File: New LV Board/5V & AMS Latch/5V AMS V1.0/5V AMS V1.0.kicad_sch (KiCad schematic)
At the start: 17 parts, among them J2 B12B-PH-K-S, J4 691137710002, K1 AHES4291, SW1 Test Reset AMS, U1 LT1117-5.0

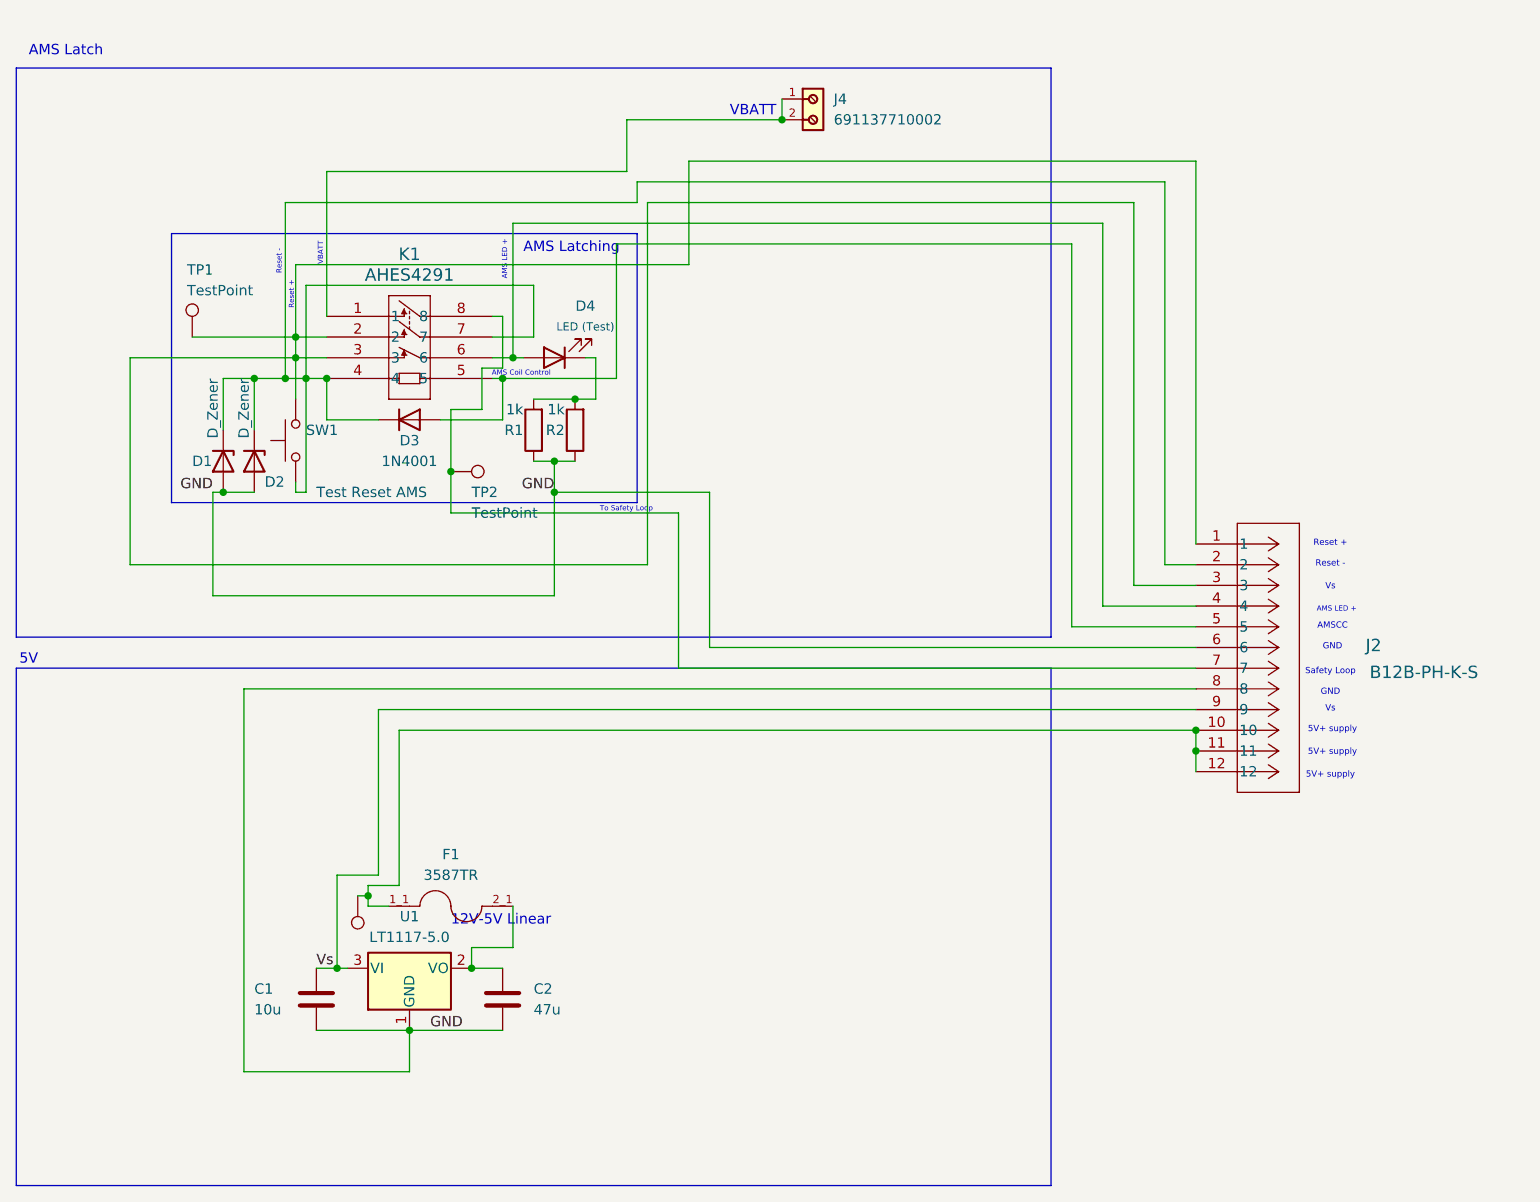
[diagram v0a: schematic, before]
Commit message: Relay wiring
Relay Wiring
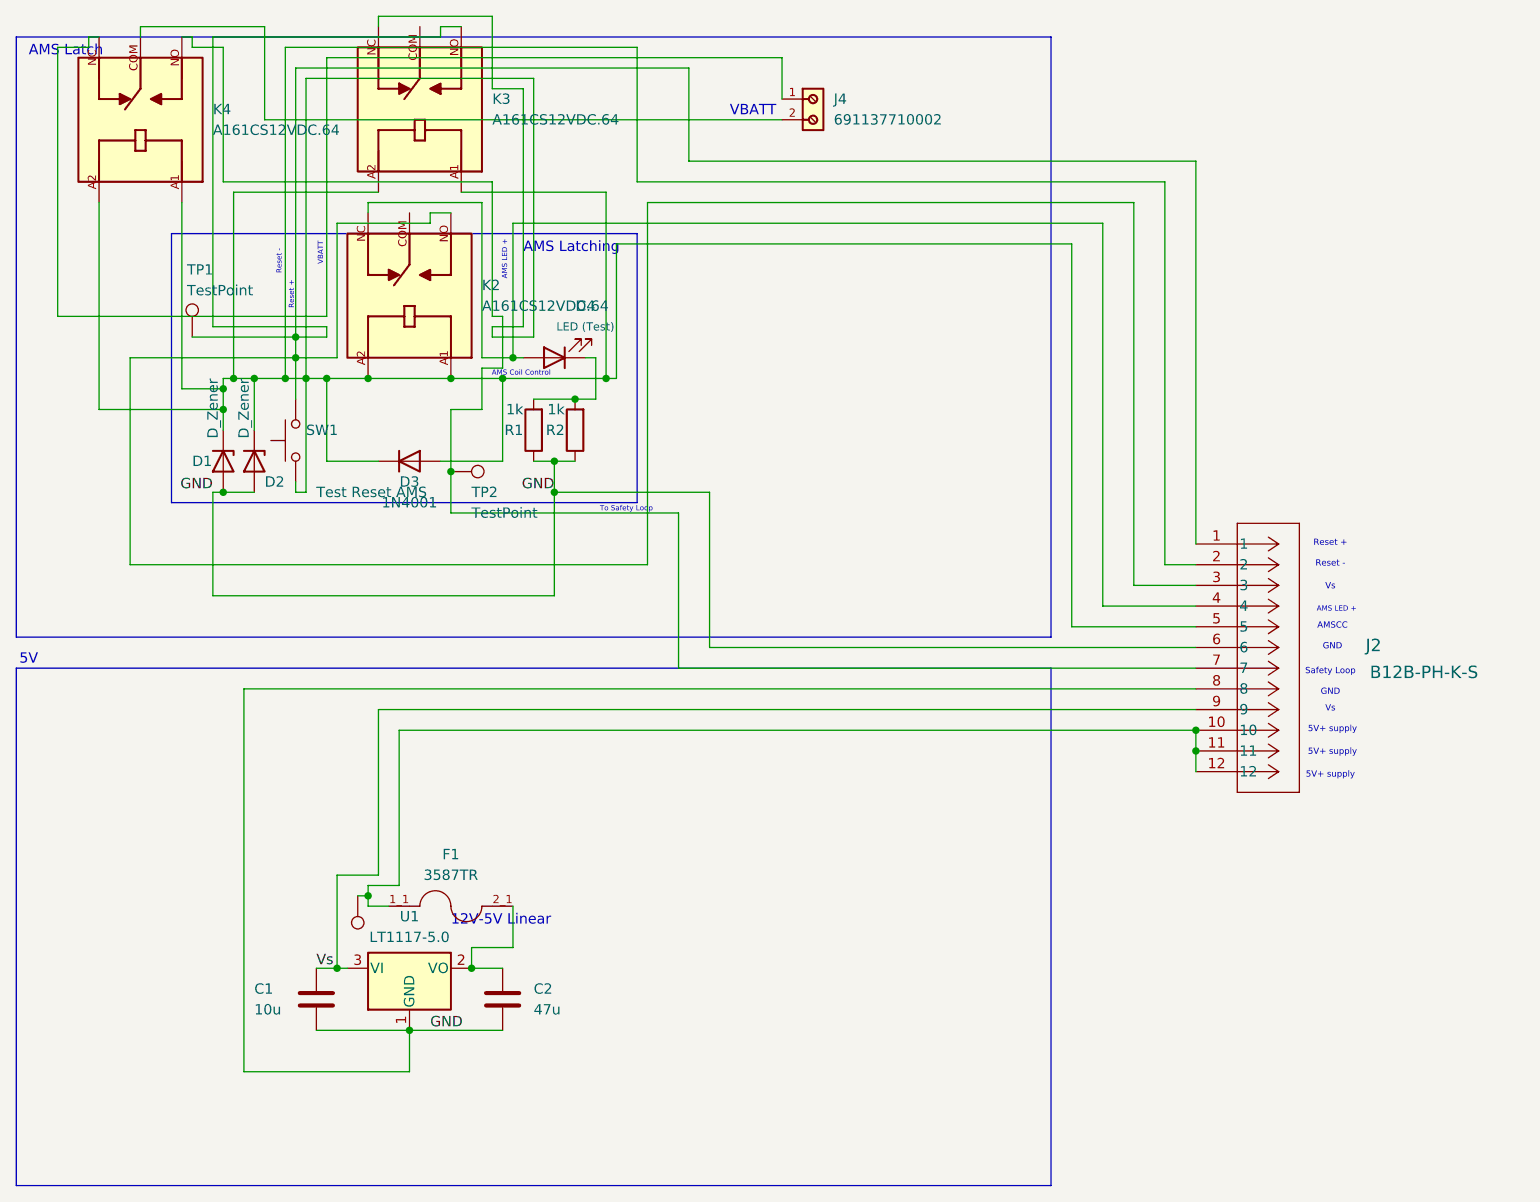
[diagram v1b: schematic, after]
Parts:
- removed K1: AHES4291, motorSports:AHES4_PAN, symbol Relay:AHES4291
- added K2, K3, K4: A161CS12VDC.64, A161CS12VDC.64:RELAY_A161CS12VDC.64, symbol A161CS12VDC.64:A161CS12VDC.64
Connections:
- net at D4.2 (A), J2.4: now also K2.NC
- net at D1.1 (K), D2.1 (K), D3.1 (K)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: now also D3.2 (A), J2.5, K2.A1, K2.A2, K3.A1, K3.A2, K3.NC, K4.A1, K4.A2
- net at J4.1: now also K4.NC; no longer J4.2
- net at J2.7, TP2.1: now also K4.NO
- net at J2.1, J2.3, SW1.2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: now also K2.NO, K3.NO
- new net: J4.2, K4.COM
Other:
- moved on the sheet: D3
